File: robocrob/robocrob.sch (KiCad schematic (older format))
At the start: 5 parts, among them J1 Conn_01x03_Female, SW2 SW_DIP_x02

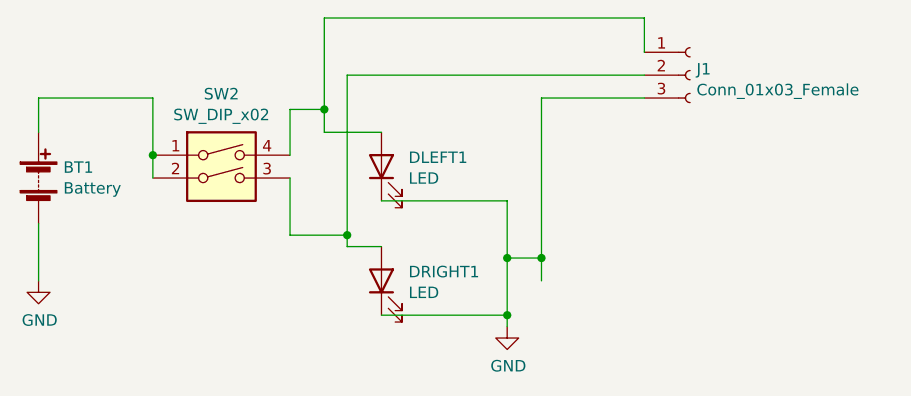
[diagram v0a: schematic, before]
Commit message: ship it or die trying
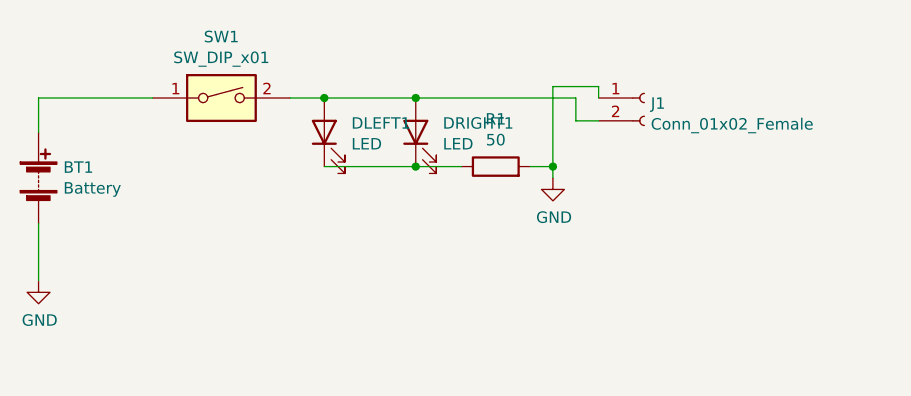
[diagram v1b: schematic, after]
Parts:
- removed J1: Conn_01x03_Female, Connector_PinHeader_2.54mm:PinHeader_1x03_P2.54mm_Vertical, symbol Connector:Conn_01x03_Female
- removed SW2: SW_DIP_x02, Button_Switch_SMD:SW_DPDT_CK_JS202011JCQN, symbol Switch:SW_DIP_x02
- added J1: Conn_01x02_Female, Connector_PinSocket_2.54mm:PinSocket_1x02_P2.54mm_Vertical, symbol Connector:Conn_01x02_Female
- added R1: 50, Resistor_SMD:R_1206_3216Metric_Pad1.42x1.75mm_HandSolder, symbol Device:R
- added SW1: SW_DIP_x01, Button_Switch_SMD:SW_DIP_SPSTx01_Slide_6.7x4.1mm_W8.61mm_P2.54mm_LowProfile, symbol Switch:SW_DIP_x01
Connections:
- wire segments 27 -> 15
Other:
- moved on the sheet: DLEFT1, DRIGHT1
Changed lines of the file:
@@
 L Device:LED DLEFT1
 U 1 1 5FCF4ABB
-P 3000 2650
-F 0 "DLEFT1" V 3039 2532 50  0000 R CNN
-F 1 "LED" V 2948 2532 50  0000 R CNN
-F 2 "LED_THT:LED_D5.0mm" H 3000 2650 50  0001 C CNN
-F 3 "~" H 3000 2650 50  0001 C CNN
-	1    3000 2650
+P 2750 2500
+F 0 "DLEFT1" V 2789 2382 50  0000 R CNN
+F 1 "LED" V 2698 2382 50  0000 R CNN
+F 2 "LED_THT:LED_D5.0mm" H 2750 2500 50  0001 C CNN
+F 3 "~" H 2750 2500 50  0001 C CNN
+	1    2750 2500
 	0    -1   -1   0
 $EndComp
@@
 L Device:LED DRIGHT1
 U 1 1 5FD0087F
-P 3000 3150
-F 0 "DRIGHT1" V 3039 3032 50  0000 R CNN
-F 1 "LED" V 2948 3032 50  0000 R CNN
-F 2 "LED_THT:LED_D5.0mm" H 3000 3150 50  0001 C CNN
-F 3 "~" H 3000 3150 50  0001 C CNN
-	1    3000 3150
+P 3150 2500
+F 0 "DRIGHT1" V 3189 2382 50  0000 R CNN
+F 1 "LED" V 3098 2382 50  0000 R CNN
+F 2 "LED_THT:LED_D5.0mm" H 3150 2500 50  0001 C CNN
+F 3 "~" H 3150 2500 50  0001 C CNN
+	1    3150 2500
 	0    -1   -1   0
 $EndComp
@@
 L power:GND #PWR0102
 U 1 1 5FD0C04D
-P 3550 3350
-F 0 "#PWR0102" H 3550 3100 50  0001 C CNN
-F 1 "GND" H 3555 3177 50  0000 C CNN
-F 2 "" H 3550 3350 50  0001 C CNN
-F 3 "" H 3550 3350 50  0001 C CNN
-	1    3550 3350
+P 3750 2700
+F 0 "#PWR0102" H 3750 2450 50  0001 C CNN
+F 1 "GND" H 3755 2527 50  0000 C CNN
+F 2 "" H 3750 2700 50  0001 C CNN
+F 3 "" H 3750 2700 50  0001 C CNN
+	1    3750 2700
 	1    0    0    -1
 $EndComp
@@
 	1500 2350 1500 2500
 Wire Wire Line
-	2750 2000 2750 2400
-Wire Wire Line
-	2750 2500 3000 2500
-Wire Wire Line
-	2850 2250 2850 2950
-Wire Wire Line
-	2850 3000 3000 3000
-Wire Wire Line
-	3700 3050 3550 3050
-Connection ~ 3550 3050
-Wire Wire Line
-	3550 3050 3550 3300
-Wire Wire Line
-	3000 2800 3550 2800
-Wire Wire Line
-	3550 2800 3550 3050
-Wire Wire Line
-	3000 3300 3550 3300
-Connection ~ 3550 3300
-Wire Wire Line
-	3550 3300 3550 3350
+	1500 2350 2000 2350
 $Comp
-L Switch:SW_DIP_x02 SW2
-U 1 1 5FD284EE
-P 2300 2700
-F 0 "SW2" H 2300 3067 50  0000 C CNN
-F 1 "SW_DIP_x02" H 2300 2976 50  0000 C CNN
-F 2 "Button_Switch_SMD:SW_DPDT_CK_JS202011JCQN" H 2300 2700 50  0001 C CNN
-F 3 "~" H 2300 2700 50  0001 C CNN
-	1    2300 2700
+L Connector:Conn_01x02_Female J1
+U 1 1 5FD3F41C
+P 4150 2350
+F 0 "J1" H 4178 2326 50  0000 L CNN
+F 1 "Conn_01x02_Female" H 4178 2235 50  0000 L CNN
+F 2 "Connector_PinSocket_2.54mm:PinSocket_1x02_P2.54mm_Vertical" H 4150 2350 50  0001 C CNN
+F 3 "~" H 4150 2350 50  0001 C CNN
+	1    4150 2350
+	1    0    0    -1
+$EndComp
+$Comp
+L Switch:SW_DIP_x01 SW1
+U 1 1 5FD3BC38
+P 2300 2350
+F 0 "SW1" H 2300 2617 50  0000 C CNN
+F 1 "SW_DIP_x01" H 2300 2526 50  0000 C CNN
+F 2 "Button_Switch_SMD:SW_DIP_SPSTx01_Slide_6.7x4.1mm_W8.61mm_P2.54mm_LowProfile" H 2300 2350 50  0001 C CNN
+F 3 "~" H 2300 2350 50  0001 C CNN
+	1    2300 2350
 	1    0    0    -1
 $EndComp
 Wire Wire Line
-	2000 2350 2000 2600
+	2600 2350 2750 2350
+Connection ~ 2750 2350
 Wire Wire Line
-	1500 2350 2000 2350
-Connection ~ 2000 2600
+	2750 2350 3150 2350
+Connection ~ 3150 2350
 Wire Wire Line
-	2000 2600 2000 2700
+	2750 2650 3150 2650
+Connection ~ 3750 2650
 Wire Wire Line
-	2600 2600 2600 2400
+	3750 2650 3750 2700
+Connection ~ 3150 2650
 Wire Wire Line
-	2600 2400 2750 2400
-Connection ~ 2750 2400
+	3150 2650 3350 2650
 Wire Wire Line
-	2750 2400 2750 2500
+	3850 2350 3850 2450
 Wire Wire Line
-	2600 2700 2600 2950
+	3850 2450 3950 2450
 Wire Wire Line
-	2600 2950 2850 2950
-Connection ~ 2850 2950
+	3150 2350 3850 2350
 Wire Wire Line
-	2850 2950 2850 3000
+	3750 2300 3950 2300
+Wire Wire Line
+	3950 2300 3950 2350
+Wire Wire Line
+	3750 2300 3750 2650
 $Comp
-L Connector:Conn_01x03_Female J1
-U 1 1 5FD2E4C7
-P 4350 2250
-F 0 "J1" H 4378 2276 50  0000 L CNN
-F 1 "Conn_01x03_Female" H 4378 2185 50  0000 L CNN
-F 2 "Connector_PinHeader_2.54mm:PinHeader_1x03_P2.54mm_Vertical" H 4350 2250 50  0001 C CNN
-F 3 "~" H 4350 2250 50  0001 C CNN
-	1    4350 2250
-	1    0    0    -1
+L Device:R R1
+U 1 1 5FD52D15
+P 3500 2650
+F 0 "R1" V 3707 2650 50  0000 C CNN
+F 1 "50" V 3616 2650 50  0000 C CNN
+F 2 "Resistor_SMD:R_1206_3216Metric_Pad1.42x1.75mm_HandSolder" V 3430 2650 50  0001 C CNN
+F 3 "~" H 3500 2650 50  0001 C CNN
+	1    3500 2650
+	0    -1   -1   0
 $EndComp
 Wire Wire Line
-	4150 2000 4150 2150
-Wire Wire Line
-	2750 2000 4150 2000
-Wire Wire Line
-	2850 2250 4150 2250
-Wire Wire Line
-	3700 2350 4150 2350
-Wire Wire Line
-	3700 2350 3700 3050
-Connection ~ 3700 3050
-Wire Wire Line
-	3700 3050 3700 3150
+	3650 2650 3750 2650
 $EndSCHEMATC
